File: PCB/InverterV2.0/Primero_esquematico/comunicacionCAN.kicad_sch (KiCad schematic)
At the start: 14 parts, among them J3 347920040, U33 ISO1042DWR, U34 ISO1042DWR

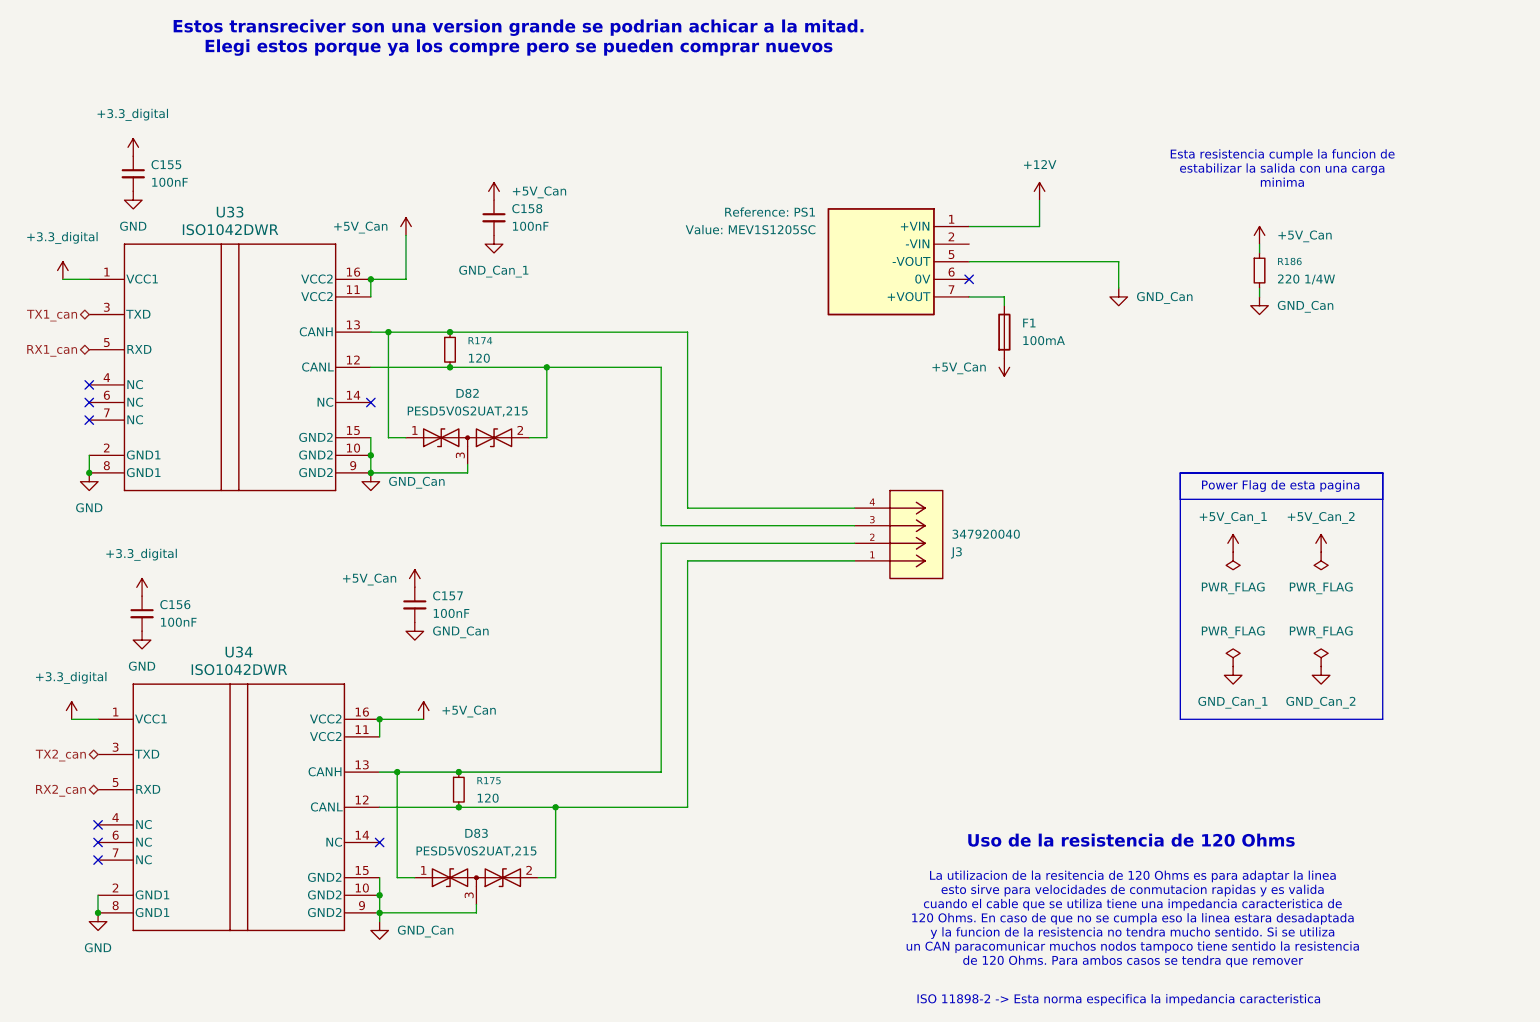
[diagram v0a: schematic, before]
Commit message: aislacion encoder
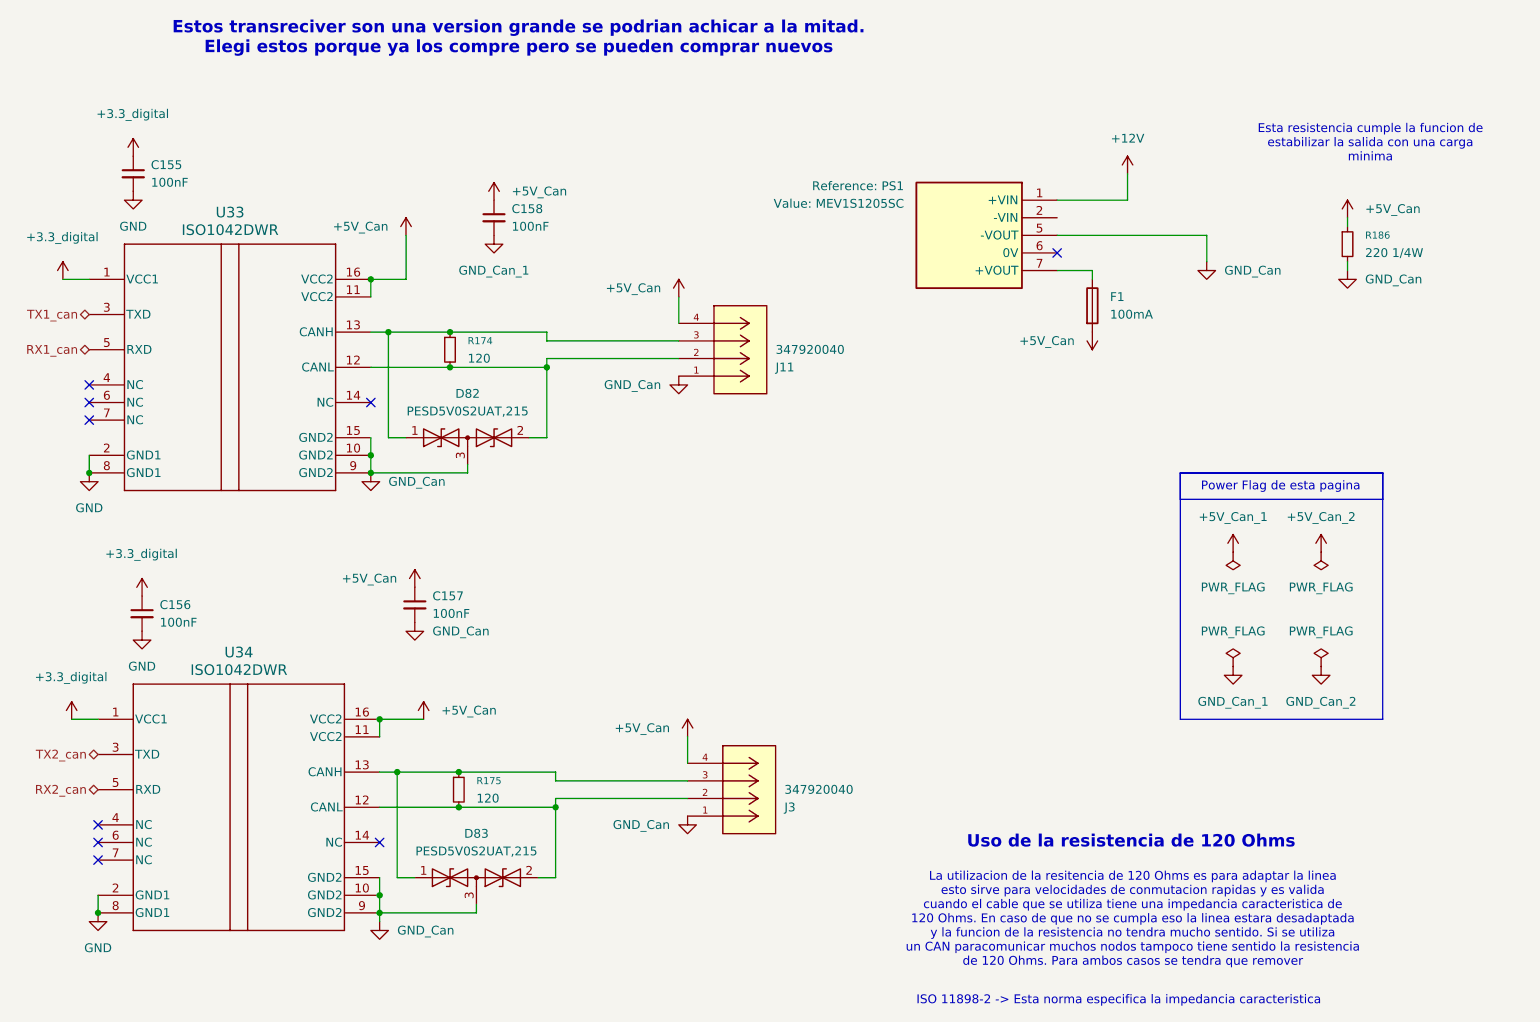
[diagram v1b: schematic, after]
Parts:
- added J11: 347920040, Snapeda:CONN04_34792_MOL, symbol Snapeda:347920040
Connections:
- net +5V_Can: now also J3.4, J11.4
- net GND_Can: now also J3.1, J11.1
- net at D82.1 (A1), R174.1, U33.13 (CANH): now also J11.3; no longer J3.4
- net at D82.2 (A2), R174.2, U33.12 (CANL): now also J11.2; no longer J3.3
- net at D83.2 (A2), R175.2, U34.12 (CANL): now also J3.2; no longer J3.1
- net at D83.1 (A1), R175.1, U34.13 (CANH): now also J3.3; no longer J3.2
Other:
- moved on the sheet: F1, R186, Reference: PS1
